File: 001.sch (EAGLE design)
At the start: 27 parts, among them CN01 PWR5V, CN02 JD-VCC, CN03 TO-RLY, CN04 I2C-LCD, CN05 INPUT-A, CN06 INPUT-B, CN07 BUTTON-A, CN08 BUTTON-B, CN09 BUTTON-STOP, CN10 DELAY-VR, M1 ARDUINO-NANO-3.0

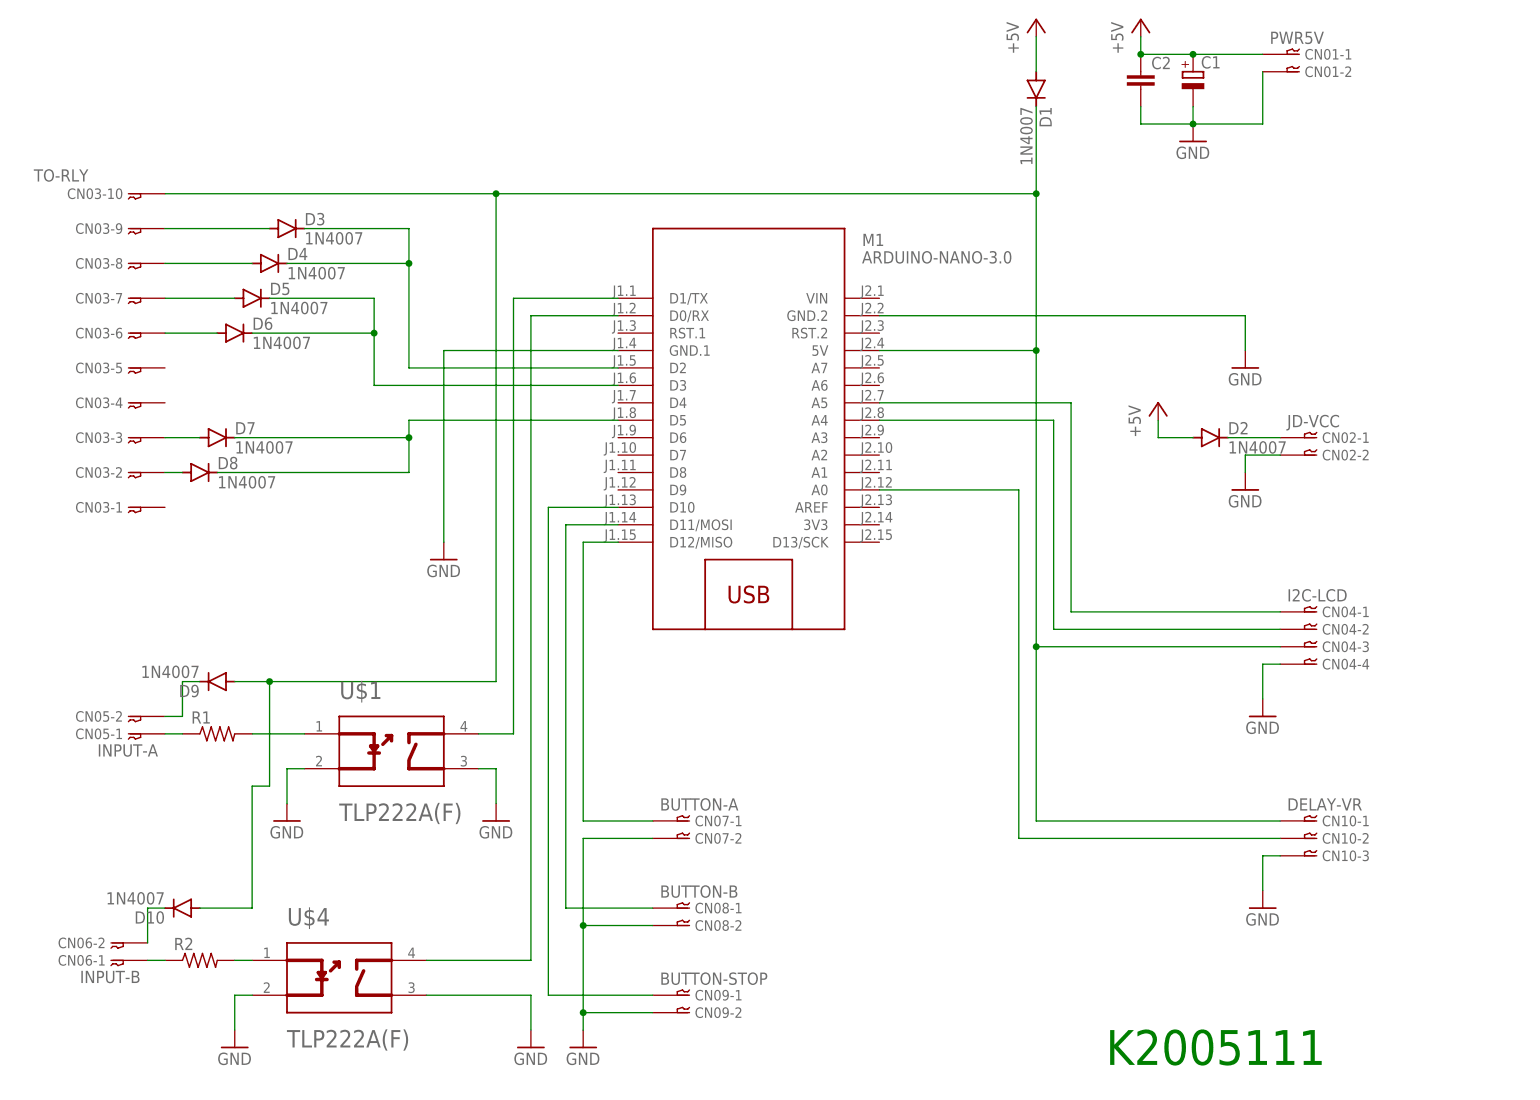
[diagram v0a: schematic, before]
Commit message: ソースコードと一緒に管理
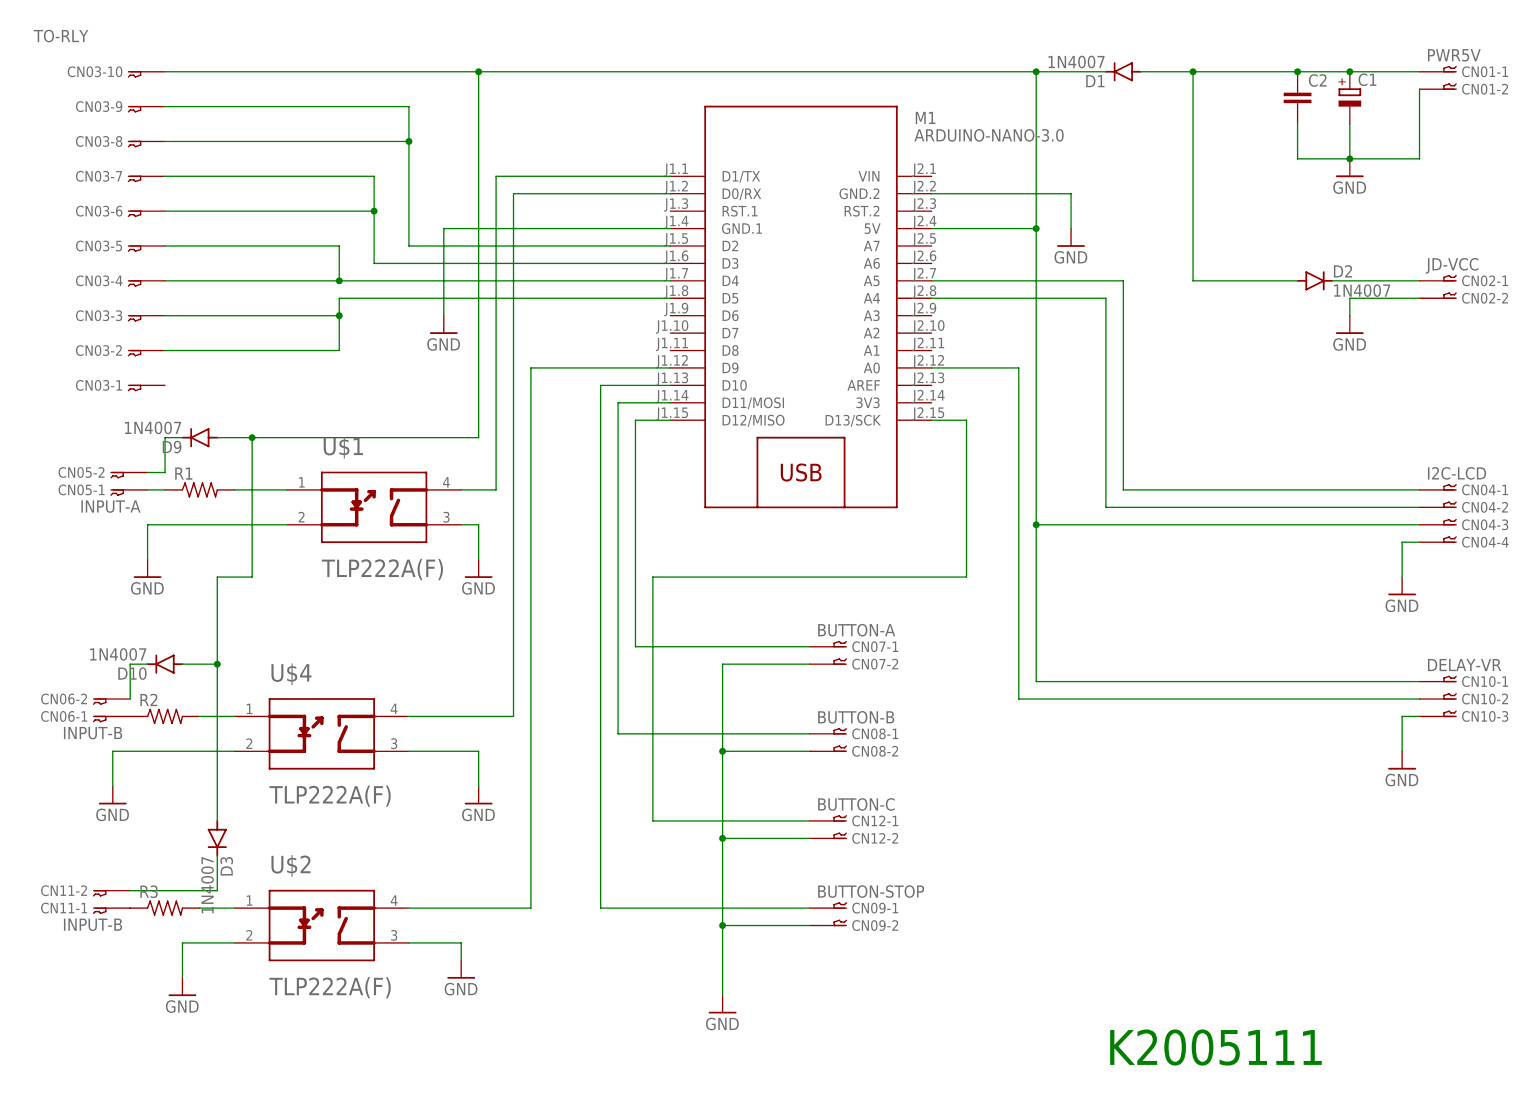
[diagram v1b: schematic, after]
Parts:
- removed D4, D5, D6, D7, D8: 1N4007, diode:1N4004
- added CN11: INPUT-B, holly:02-JST-A
- added CN12: BUTTON-C, holly:02-JST-A
- added R3: (no value), rcl:R-US_0207/7
- added U$2: (no value), Toshiba-TLP222AF:TOSHIBA_TLP222A_F_SIMPLE
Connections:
- net +5V renamed N$10
- removed net N$10 (its old number): CN03-2.1, D8.A
- removed net N$15: D7.C, D8.C, M1.D5
- new net N$1: CN03-4.1, CN03-5.1, M1.D4
- new net N$12: CN11-2.1, D3.C
- net 5V: now also D3.A
- net GND: now also CN12-2.1, U$2.1_DRAIN, U$2.CATHODE
- net N$11: now also CN03-6.1, CN03-7.1; no longer D5.C, D6.C
- net N$14: now also CN03-8.1, CN03-9.1; no longer D3.C, D4.C
- net N$3: now also CN03-2.1, CN03-3.1, M1.D5; no longer CN03-9.1, D3.A
- net N$6: now also M1.D9, U$2.2_DRAIN; no longer CN03-8.1, D4.A
- net N$7: now also CN11-1.1, R3.1; no longer CN03-7.1, D5.A
- net N$8: now also R3.2, U$2.ANODE; no longer CN03-6.1, D6.A
- net N$9: now also CN12-1.1, M1.D13/SCK; no longer CN03-3.1, D7.A
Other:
- moved on the sheet: C1, C2, CN01-1, CN01-2, CN02-1, CN02-2, CN03-1, CN03-10, CN03-2, CN03-3, CN03-4, CN03-5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
